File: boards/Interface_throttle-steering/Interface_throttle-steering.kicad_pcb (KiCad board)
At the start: 2 copper layers, 69.8 x 54.2 mm, 5 parts, among them J1 micromatch_male_4, J2 Ultrafit_4, J3 micromatch_male_20, J4 Ampseal_23, U1 RJ45

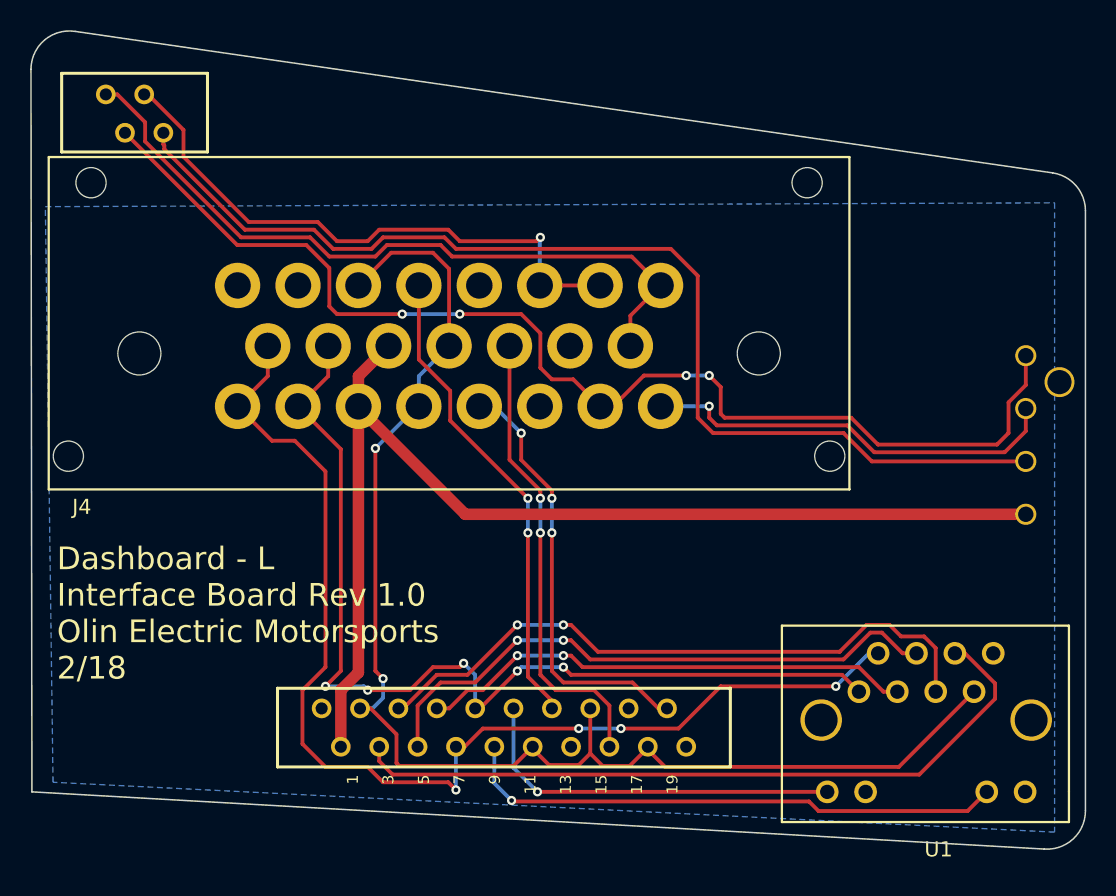
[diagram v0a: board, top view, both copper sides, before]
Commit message: Rev 2 files for throttle-steering
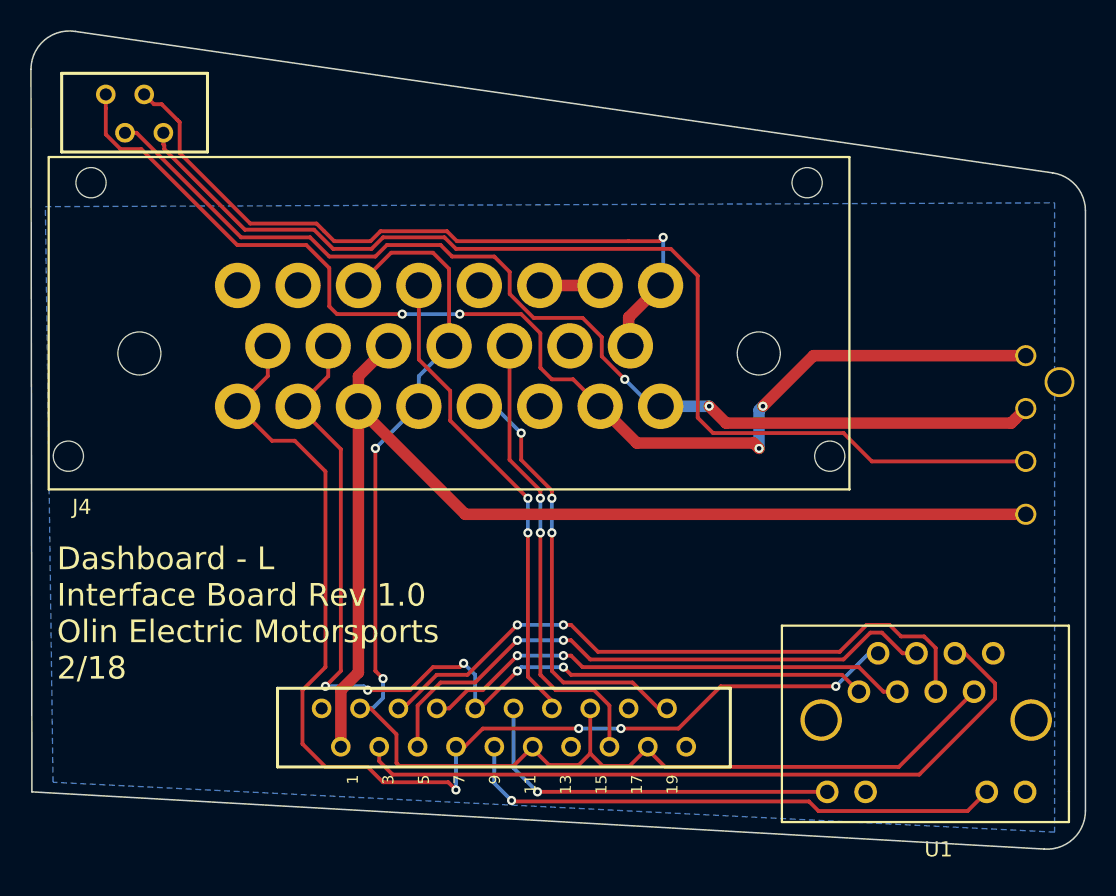
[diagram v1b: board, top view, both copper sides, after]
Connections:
- J1 pad 1: /BOTS_sense -> /BOTS_In/E-Stop_Out
- J1 pad 2: /BOTS_In/E-Stop_Out -> /E-Stop_In/Connector_to_HVD_Out
- J1 pad 3: /BSPD_In/Crash_Sensor_Out -> /Crash_Sensor_In/BOTS_Out
- J4 pad 15: /BOTS_sense -> /Crash_Sensor_In/BOTS_Out
- J4 pad 8: /BOTS_sense -> /Crash_Sensor_In/BOTS_Out
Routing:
- net /Crash_Sensor_In/BOTS_Out: track 0.00 -> 48.4 mm, vias 0 -> 1
- net /BOTS_sense: track 48.2 -> 0.00 mm
- net /E-Stop_In/Connector_to_HVD_Out: track 28.0 -> 70.2 mm, vias 1 -> 2
- net /BSPD_In/Crash_Sensor_Out: track 39.2 -> 4.21 mm, vias 1 -> 0
- net /BOTS_In/E-Stop_Out: track 78.5 -> 79.9 mm
